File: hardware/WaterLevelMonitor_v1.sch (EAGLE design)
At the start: 43 parts, among them J1 D24V5F5, J2 AVR_SPI_PRG_6PTH, J5 D24V5F5, J6 D24V5F5, J7 RJ45, Q1 NDP6020P, Q4 2N3904, U1 ATMEGA328P_PDIP

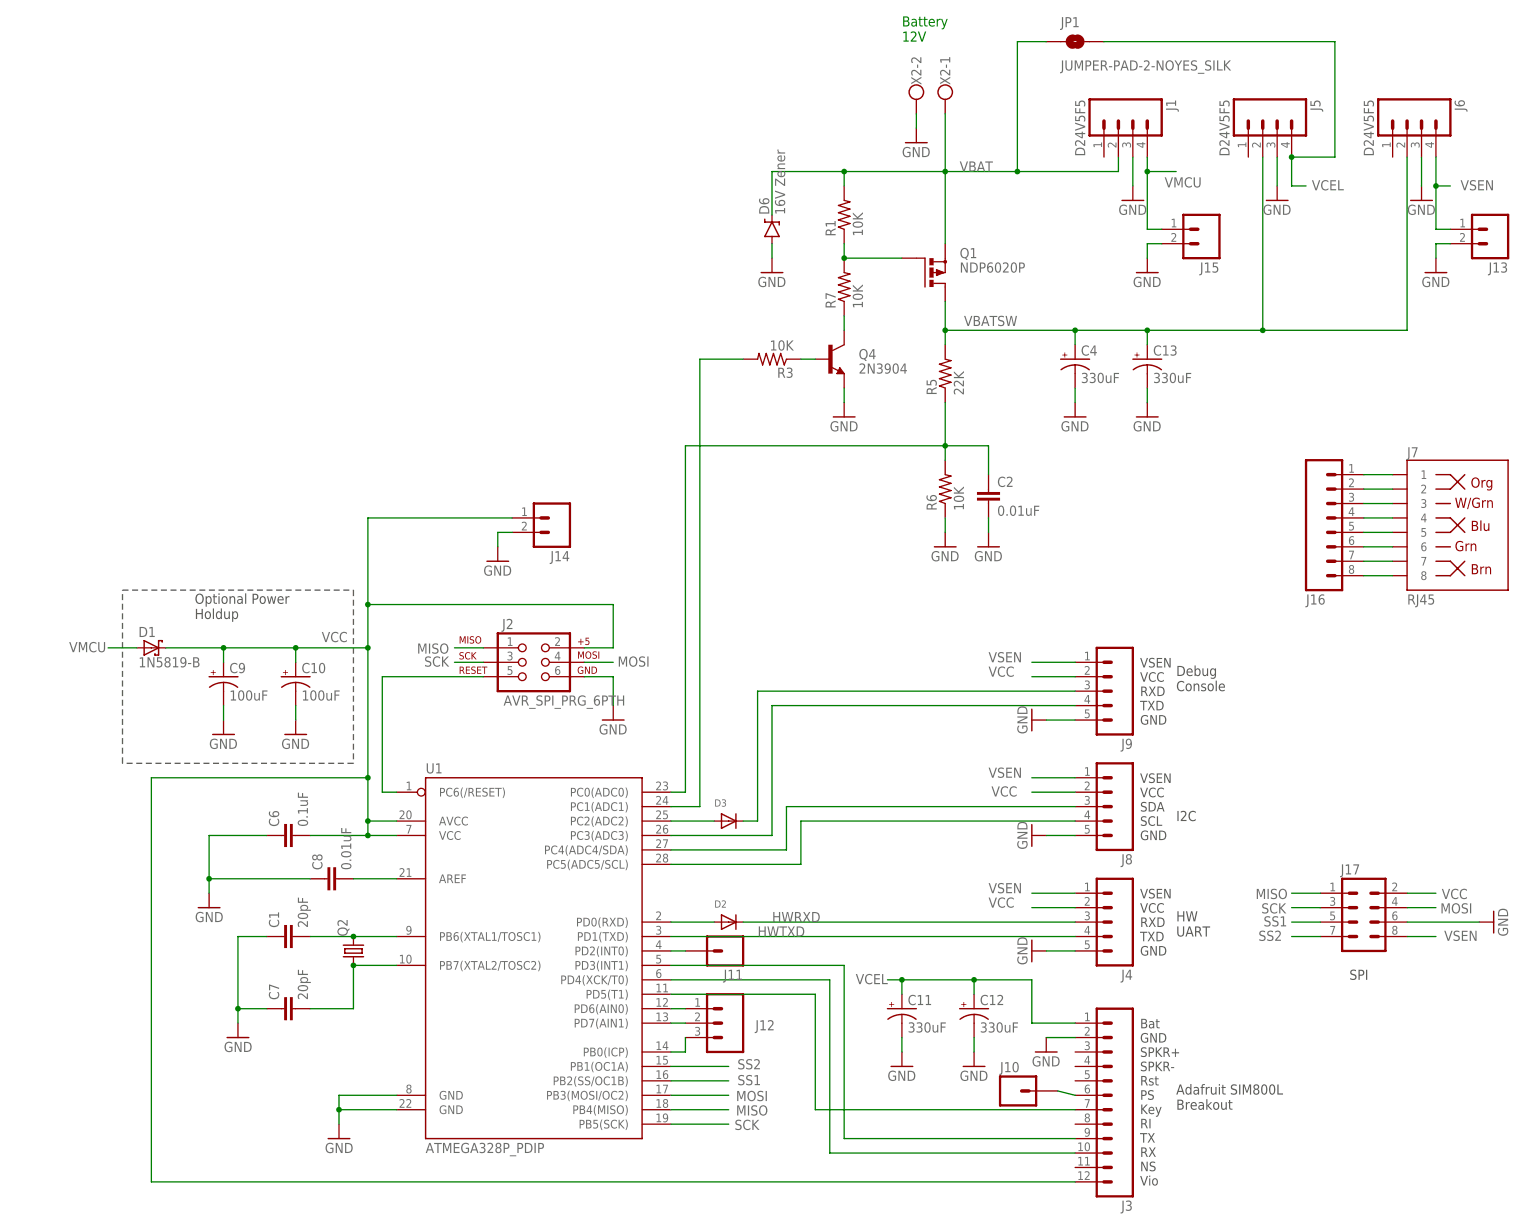
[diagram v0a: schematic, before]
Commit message: Add files via upload
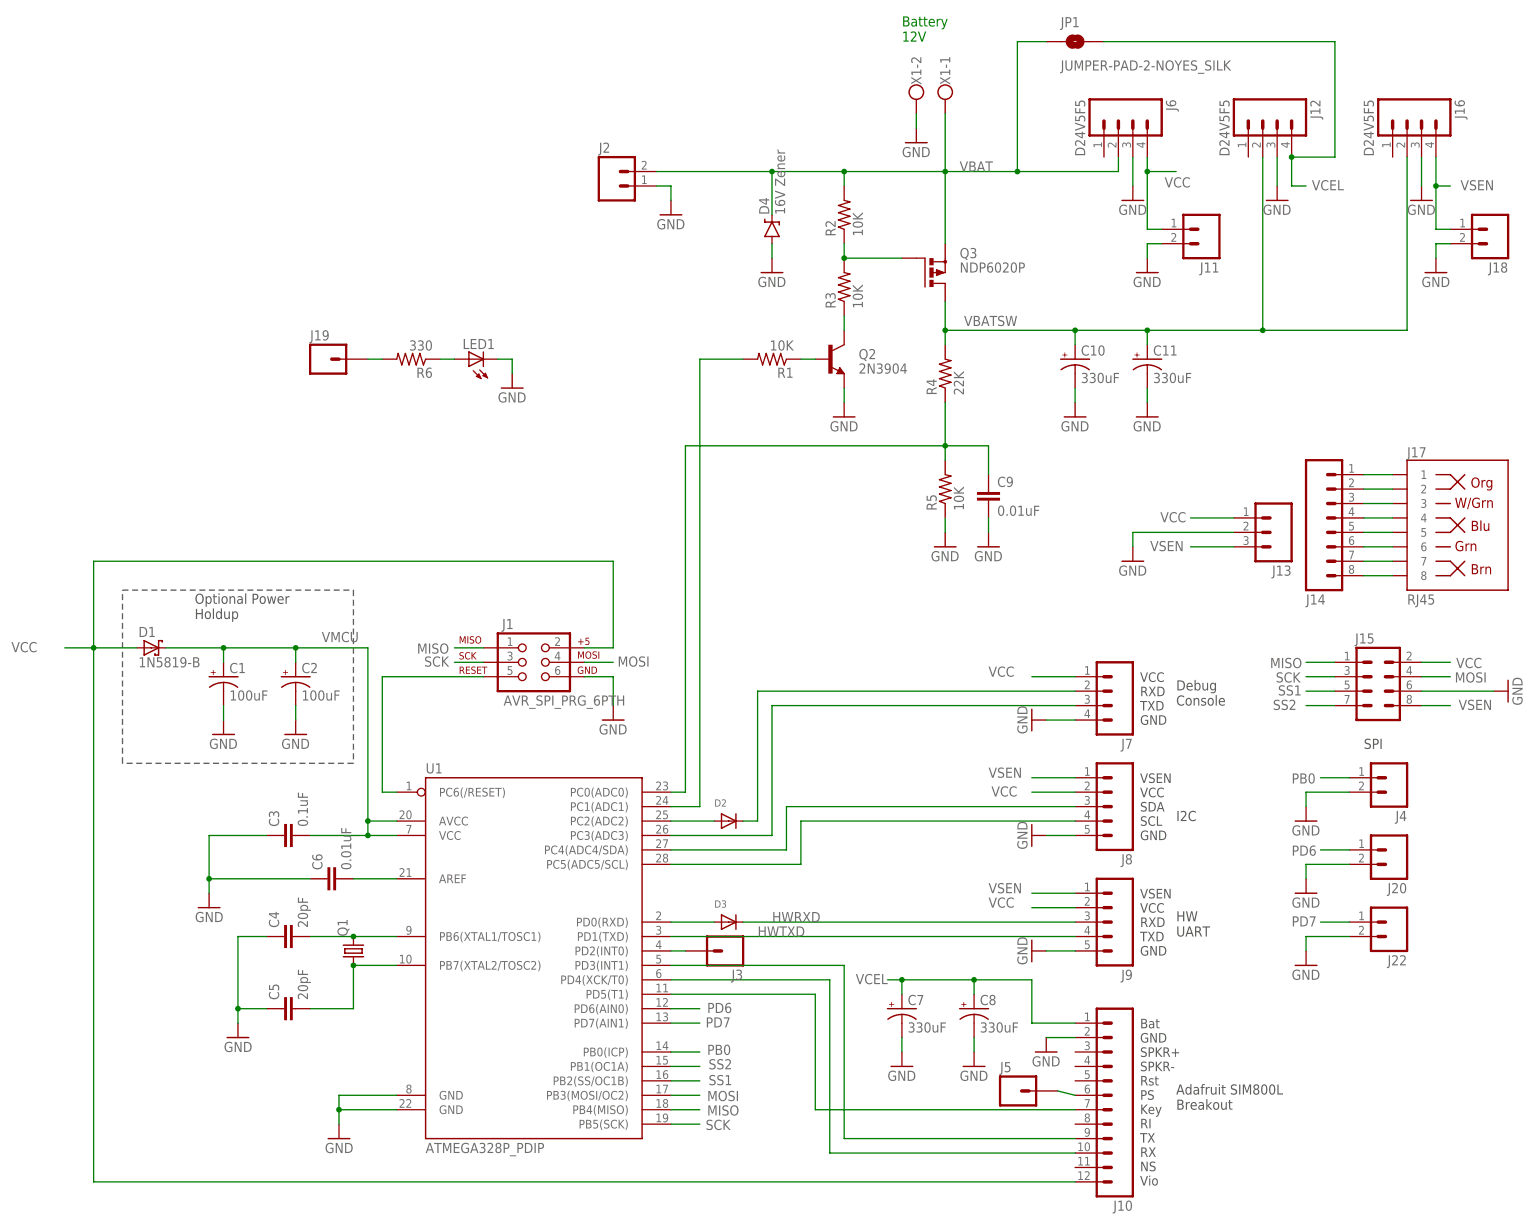
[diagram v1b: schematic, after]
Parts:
- removed C12, C13: 330uF, SparkFun-Capacitors:CAP_POLPTH1
- removed Q4: 2N3904, SparkFun-DiscreteSemi:TRANSISTOR_NPNTO-92-AMMO
- removed R7: 10K, resistor:R-US_0204/5
- added C3: 0.1uF, SparkFun-Capacitors:CAPPTH
- added C5: 20pF, SparkFun-Capacitors:CAPPTH
- added J18: (no value), SparkFun-Connectors:M02PTH
- added J19: (no value), SparkFun-Connectors:M01PTH_NO_SILK_YES_STOP
- added J20, J22: (no value), SparkFun-Connectors:M021X02_NO_SILK
- added LED1: (no value), led:LED5MM
- added Q3: NDP6020P, transistor-power:PMOSFET_PTO220BV
- added R2: 10K, resistor:R-US_0204/5
- added R4: 22K, resistor:R-US_0204/5
- C1: value 20pF -> 100uF; device SparkFun-Capacitors:CAPPTH -> SparkFun-Capacitors:CAP_POLPTH1
- C10: value 100uF -> 330uF
- C2: value 0.01uF -> 100uF; device SparkFun-Passives:CAPPTH1 -> SparkFun-Capacitors:CAP_POLPTH1
- C4: value 330uF -> 20pF; device SparkFun-Capacitors:CAP_POLPTH1 -> SparkFun-Capacitors:CAPPTH
- C6: value 0.1uF -> 0.01uF; device SparkFun-Capacitors:CAPPTH -> SparkFun-Passives:CAPPTH1
- C7: value 20pF -> 330uF; device SparkFun-Capacitors:CAPPTH -> SparkFun-Capacitors:CAP_POLPTH1
- C8: value 0.01uF -> 330uF; device SparkFun-Passives:CAPPTH1 -> SparkFun-Capacitors:CAP_POLPTH1
- C9: value 100uF -> 0.01uF; device SparkFun-Capacitors:CAP_POLPTH1 -> SparkFun-Passives:CAPPTH1
- J1: value D24V5F5 -> AVR_SPI_PRG_6PTH; device SparkFun-Connectors:M04PTH -> SparkFun-Connectors:AVR_SPI_PRG_6PTH
- J10: device SparkFun-Connectors:M01PTH_NO_SILK_YES_STOP -> SparkFun-Connectors:M12PTH
- J11: device SparkFun-Connectors:M01PTH_NO_SILK_YES_STOP -> SparkFun-Connectors:M02PTH
- J12: value (none) -> D24V5F5; device SparkFun-Connectors:M031X03_NO_SILK -> SparkFun-Connectors:M04PTH
- J13: device SparkFun-Connectors:M02PTH -> SparkFun-Connectors:M03PTH
- J14: device SparkFun-Connectors:M02PTH -> SparkFun-Connectors:M08SILK_FEMALE_PTH
- J15: device SparkFun-Connectors:M02PTH -> SparkFun-Connectors:M04X2
- J16: value (none) -> D24V5F5; device SparkFun-Connectors:M08SILK_FEMALE_PTH -> SparkFun-Connectors:M04PTH
- J17: value (none) -> RJ45; device SparkFun-Connectors:M04X2 -> SparkFun-Connectors:RJ45-8PTH
- J2: value AVR_SPI_PRG_6PTH -> (none); device SparkFun-Connectors:AVR_SPI_PRG_6PTH -> SparkFun-Connectors:M02PTH
- J3: device SparkFun-Connectors:M12PTH -> SparkFun-Connectors:M01PTH_NO_SILK_YES_STOP
- J4: device SparkFun-Connectors:M05PTH -> SparkFun-Connectors:M021X02_NO_SILK
- J5: value D24V5F5 -> (none); device SparkFun-Connectors:M04PTH -> SparkFun-Connectors:M01PTH_NO_SILK_YES_STOP
- J7: value RJ45 -> (none); device SparkFun-Connectors:RJ45-8PTH -> SparkFun-Connectors:M04PTH
- Q1: value NDP6020P -> (none); device transistor-power:PMOSFET_PTO220BV -> crystal:CRYSTALHC49U-V
- Q2: value (none) -> 2N3904; device crystal:CRYSTALHC49U-V -> SparkFun-DiscreteSemi:TRANSISTOR_NPNTO-92-AMMO
- R5: value 22K -> 10K
- R6: value 10K -> 330
- renumbered D6 to D4, X2 to X1
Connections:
- removed net N$37: J12.2, U1.PD7(AIN1)
- removed net N$38: J12.3, U1.PB0(ICP)
- new net N$12: LED1.A, R6.1
- new net PB0: J4.1, U1.PB0(ICP)
- new net PD6: J20.1, U1.PD6(AIN0)
- new net PD7: J22.1, U1.PD7(AIN1)
- net GND: now also C1.-, C2.-, C3.1, C4.1, C5.1, C7.-, C8.-, C9.2, J1.6, J10.2, J11.2, J12.3, J15.6, J16.3, J18.2, J2.1, J20.2, J22.2, J4.2, J7.4, LED1.C, Q2.E, R5.1; no longer C1.1, C12.-, C13.-, C2.2, C4.-, C7.1, C8.1, C9.-, J1.3, J14.2, J15.2, J17.6, J2.6, J3.2, J4.5, J5.3, Q4.E, R6.1
- net HWRXD: now also D3.C, J9.3; no longer D2.C, J4.3
- net HWTXD: now also J9.4; no longer J4.4
- net MISO: now also J1.1, J15.1; no longer J17.1, J2.1
- net MOSI: now also J1.4, J15.4; no longer J17.4, J2.4
- net N$1: now also J10.7; no longer J3.7
- net N$10: now also C5.2, Q1.1; no longer C7.2, Q2.1
- net N$11: now also C6.2; no longer C8.2
- net N$13: now also J10.6, J5.1; no longer J10.1, J3.6
- net N$14: now also Q2.C, R3.1; no longer Q4.C, R7.1
- net N$15: now also D3.A; no longer D2.A
- net N$19: now also R1.2; no longer R3.2
- net N$2: now also Q3.G, R2.1, R3.2; no longer Q1.G, R1.1, R7.2
- net N$20: now also D2.A; no longer D3.A
- net N$21: now also D2.C, J7.2; no longer D3.C, J9.3
- net N$22: now also J7.3; no longer J9.4
- net N$27: now also J14.1, J17.1; no longer J16.1, J7.1
- net N$28: now also J14.2, J17.2; no longer J16.2, J7.2
- net N$29: now also J14.3, J17.3; no longer J16.3, J7.3
- net N$3: now also Q2.B, R1.1; no longer Q4.B, R3.1
- net N$30: now also J14.4, J17.4; no longer J16.4, J7.4
- net N$31: now also J14.5, J17.5; no longer J16.5, J7.5
- net N$32: now also J1.5; no longer J2.5
- net N$33: now also J14.6, J17.6; no longer J16.6, J7.6
- net N$34: now also J14.7, J17.7; no longer J16.7, J7.7
- net N$35: now also J14.8, J17.8; no longer J16.8, J7.8
- net N$4: now also J10.9; no longer J3.9
- net N$5: now also J3.1; no longer J11.1
- net N$6: now also C9.1, R4.1, R5.2; no longer C2.1, R5.1, R6.2
- net N$7: now also J10.10; no longer J3.10
- net N$8: now also J19.1, R6.2; no longer J12.1, U1.PD6(AIN0)
- net N$9: now also C4.2, Q1.2; no longer C1.2, Q2.2
- net SCK: now also J1.3, J15.3; no longer J17.3, J2.3
- net SS1: now also J15.5; no longer J17.5
- net SS2: now also J15.7; no longer J17.7
- net VBAT: now also J2.2, J6.2, Q3.S, R2.2; no longer J1.2, Q1.S, R1.2
- net VBATSW: now also C10.+, C11.+, J12.2, J16.2, Q3.D, R4.2; no longer C13.+, C4.+, J5.2, J6.2, Q1.D, R5.2
- net VCC: now also D1.A, J1.2, J10.12, J11.1, J13.1, J15.2, J6.4, J7.1; no longer C10.+, C6.2, C9.+, D1.C, J14.1, J17.2, J2.2, J3.12, J4.2, U1.AVCC, U1.VCC
- net VCEL: now also C7.+, C8.+, J10.1, J12.4; no longer C11.+, C12.+, J3.1, J5.4
- net VMCU: now also C1.+, C2.+, C3.2, D1.C, U1.AVCC, U1.VCC; no longer D1.A, J1.4, J15.1
- net VSEN: now also J13.3, J15.8, J16.4, J18.1; no longer J13.1, J17.8, J4.1, J6.4
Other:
- note added: "VCC RXD TXD GND"
- moved on the sheet: C10, C11, C6, D2, D3, J6, J9, R1, R3, R5, R6
